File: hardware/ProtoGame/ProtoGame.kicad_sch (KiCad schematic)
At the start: 27 parts, among them J1 SD_Card_Module, SW1 SW_DPST_x2, SW10 SW_MEC_5E, SW2 SW_MEC_5E, SW3 SW_MEC_5E, SW4 SW_MEC_5E, SW5 SW_MEC_5E, SW6 SW_MEC_5E, SW7 SW_MEC_5E, SW8 SW_MEC_5E, SW9 SW_MEC_5E, U1 STM32F103C6Tx - MODULE

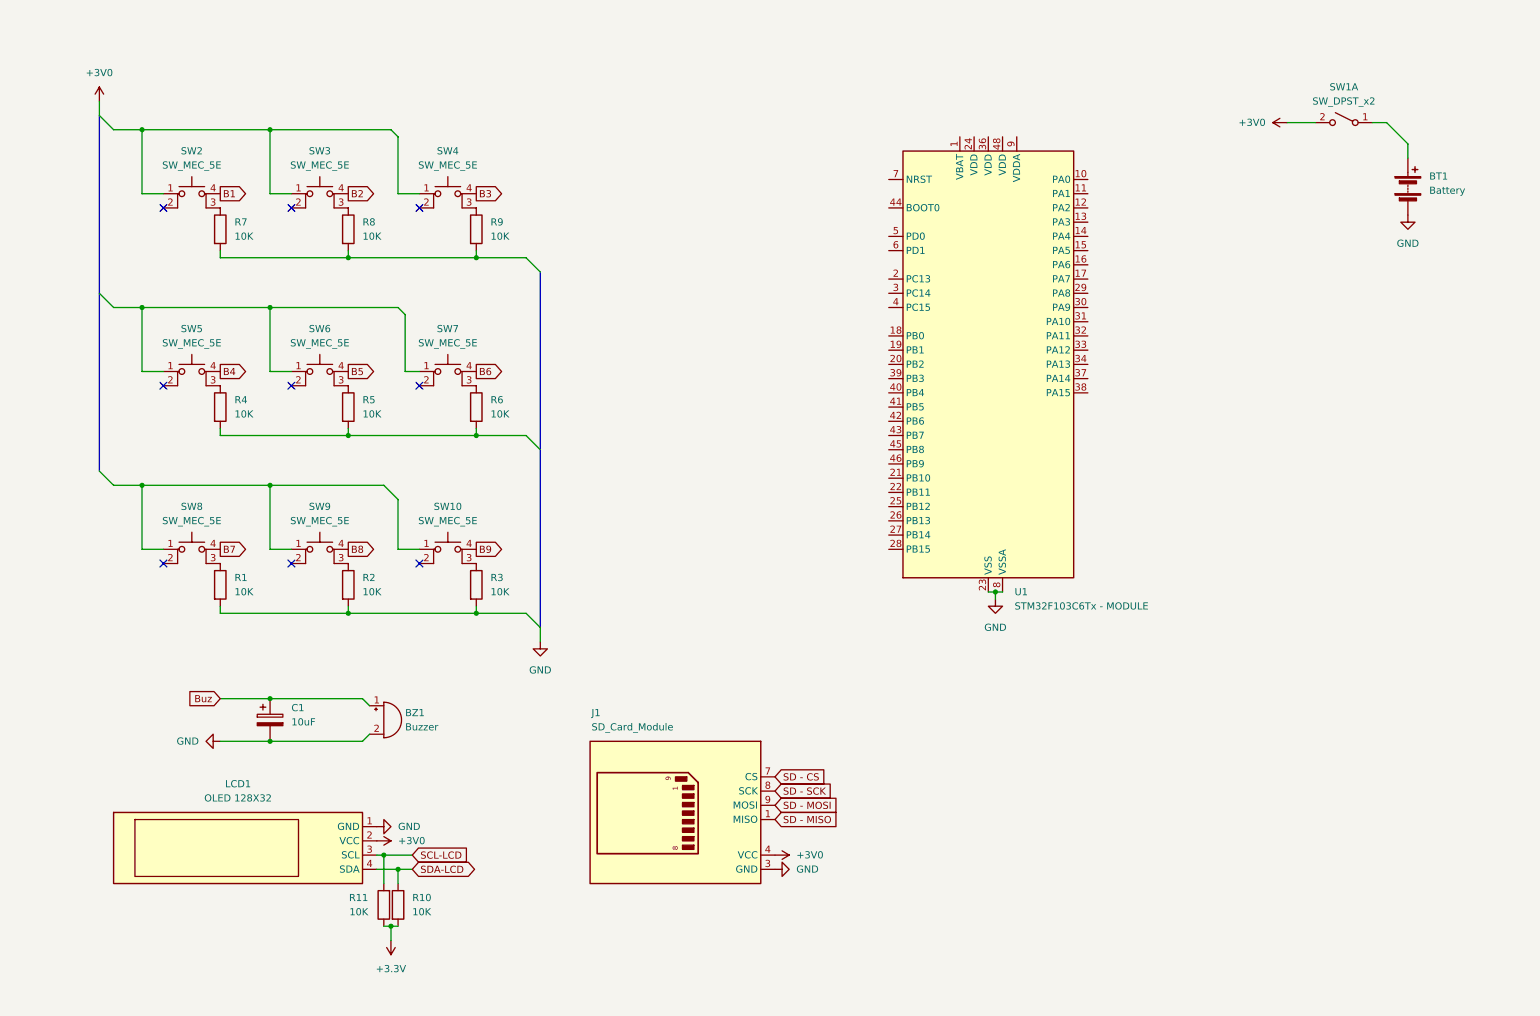
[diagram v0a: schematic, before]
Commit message: Update schemmatic
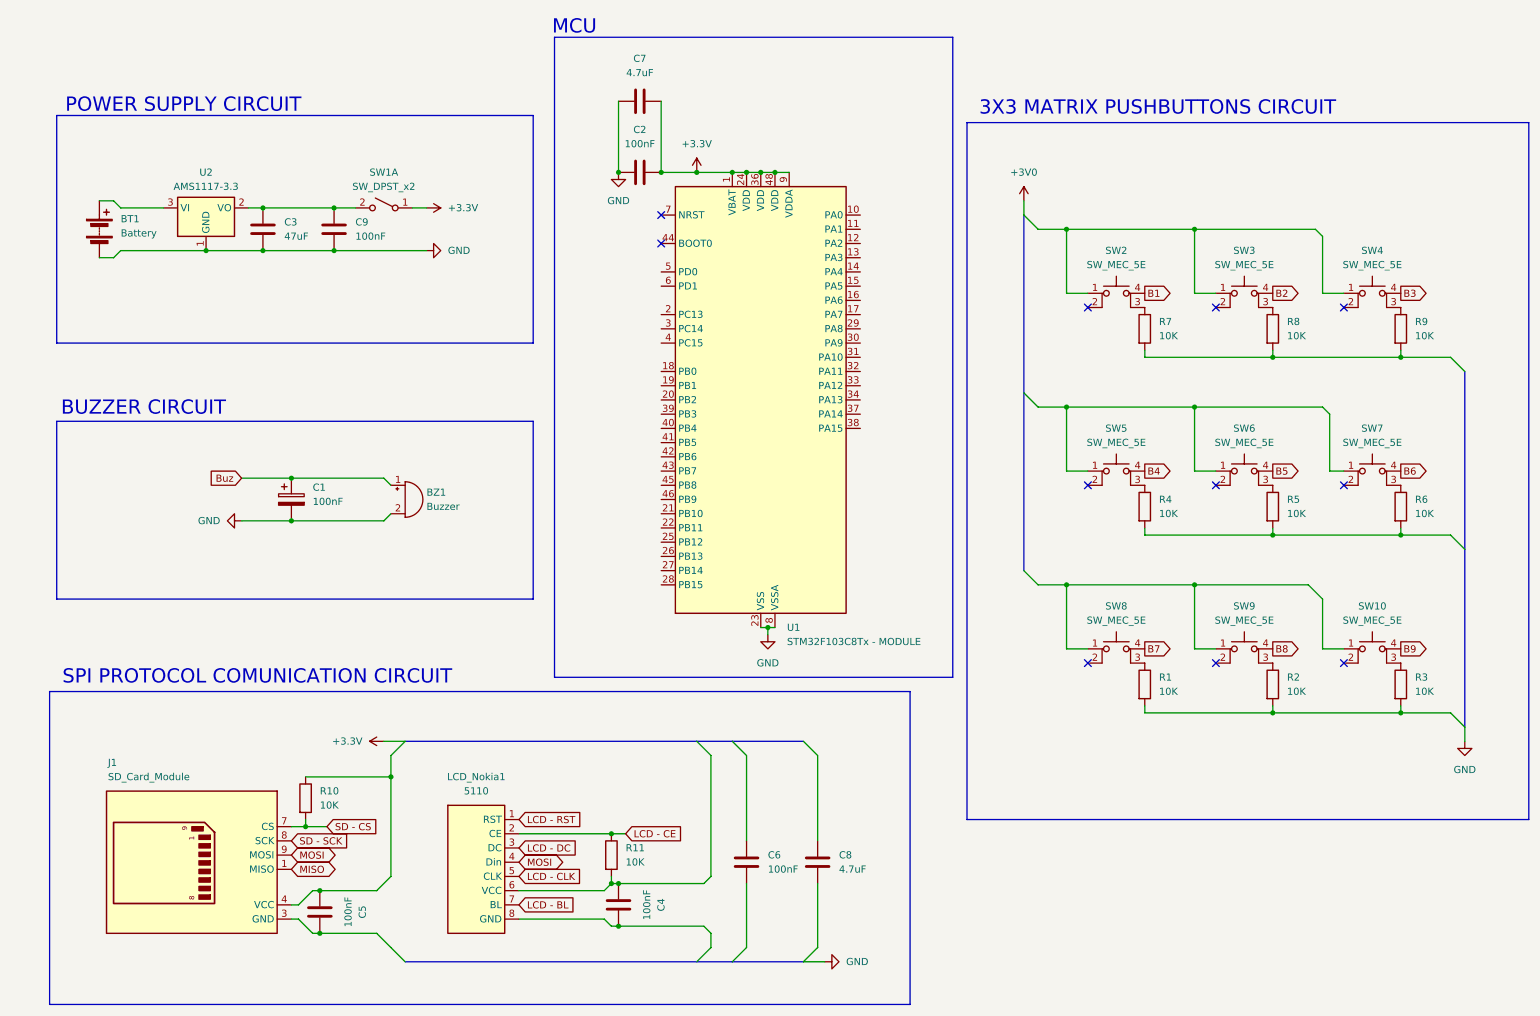
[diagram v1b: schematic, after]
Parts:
- removed LCD1: OLED 128X32, symbol LCD_Oled:LCD
- removed U1: STM32F103C6Tx - MODULE, Package_QFP:LQFP-48_7x7mm_P0.5mm, symbol MCU_ST_STM32F1:STM32F103C6Tx
- added C2, C4, C5, C6, C9: 100nF, symbol Device:C
- added C3: 47uF, symbol Device:C
- added C7, C8: 4.7uF, symbol Device:C
- added LCD_Nokia1: 5110, symbol LCD_NOKIA-5110:LCD_Nokia_5110
- added U1: STM32F103C8Tx - MODULE, Package_QFP:LQFP-48_7x7mm_P0.5mm, symbol MCU_ST_STM32F1:STM32F103C8Tx
- added U2: AMS1117-3.3, Package_TO_SOT_SMD:SOT-223-3_TabPin2, symbol Regulator_Linear:AMS1117-3.3
- C1: value 10uF -> 100nF
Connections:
- net +3.3V: now also SW1.1 (A), C2.1, C7.1, U1.1 (VBAT), U1.24 (VDD), U1.36 (VDD), U1.48 (VDD), U1.9 (VDDA); no longer R10.2, R11.1
- net +3V0: no longer J1.4 (VCC), SW1.2 (B)
- net GND: now also C2.2, C3.2, C7.2, C9.2, U1.23 (VSS), U1.35 (VSS), U1.47 (VSS), U1.8 (VSSA), U2.1 (GND); no longer J1.3 (GND)
- net SD - CS: now also R10.2
- net at BT1.1 (+): now also U2.3 (VI); no longer SW1.1 (A)
- net SCL-LCD: no longer names the net of R11.2
- net SCL-LCD: now also C4.1, LCD_Nokia1.6 (VCC)
- net SD - MISO renamed MISO
- net SD - MOSI renamed MOSI
- net MOSI: now also LCD_Nokia1.4 (Din)
- net SDA-LCD: no longer names the net of R10.1
- net SDA-LCD: now also J1.4 (VCC), C5.1
- new net: C3.1, C9.1, SW1.2 (B), U2.2 (VO)
- new net: C4.2, LCD_Nokia1.8 (GND)
- new net: C5.2, J1.3 (GND)
- new net LCD - BL: LCD_Nokia1.7 (BL)
- new net LCD - CE: LCD_Nokia1.2 (CE), R11.1
- new net LCD - CLK: LCD_Nokia1.5 (CLK)
- new net LCD - DC: LCD_Nokia1.3 (DC)
- new net LCD - RST: LCD_Nokia1.1 (RST)
- no-connect marks 9 -> 11
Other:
- note added: "3X3 MATRIX PUSHBUTTONS CIRCUIT"
- note added: "BUZZER CIRCUIT"
- note added: "MCU"
- note added: "POWER SUPPLY CIRCUIT"
- note added: "SPI PROTOCOL COMUNICATION CIRCUIT"
- moved on the sheet: BT1, BZ1, C1, J1, R1, R2, R3, R4, R5, R6, R7, R8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
